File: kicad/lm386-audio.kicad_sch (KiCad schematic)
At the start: 34 parts, among them J3 Gain, J4 Audio_IN, J5 USB, J6 Headphones, M1 TP4056_MODULE, Q1 AO3407, U1 LM386, U2 SD6271 Step Up

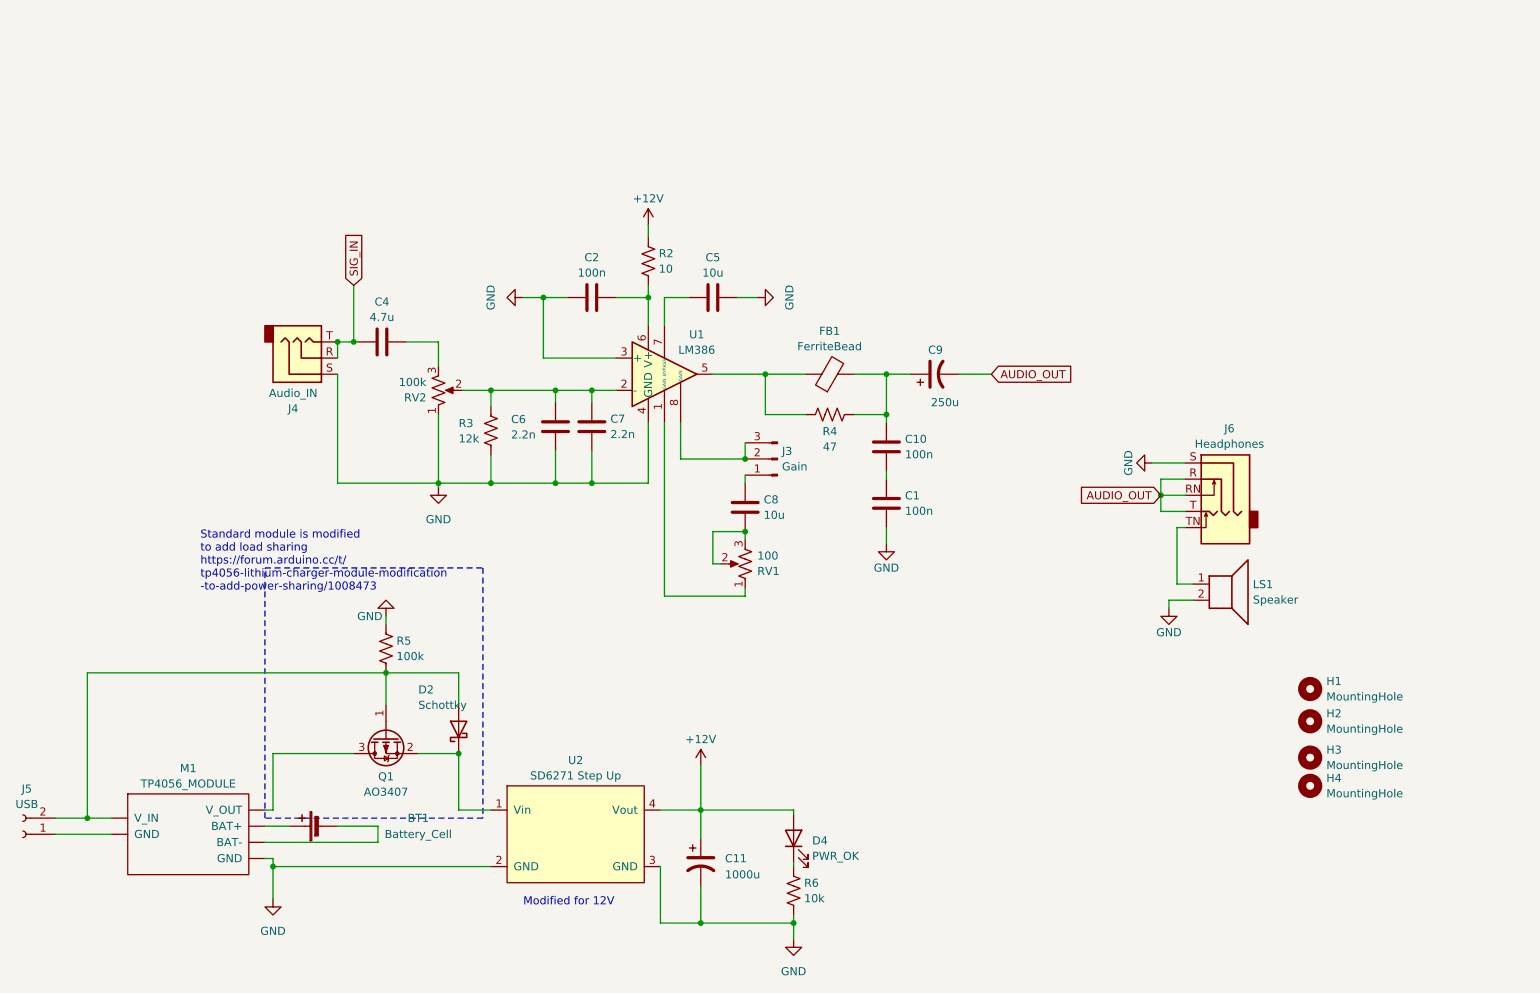
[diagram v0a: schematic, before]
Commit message: clean up + documentation
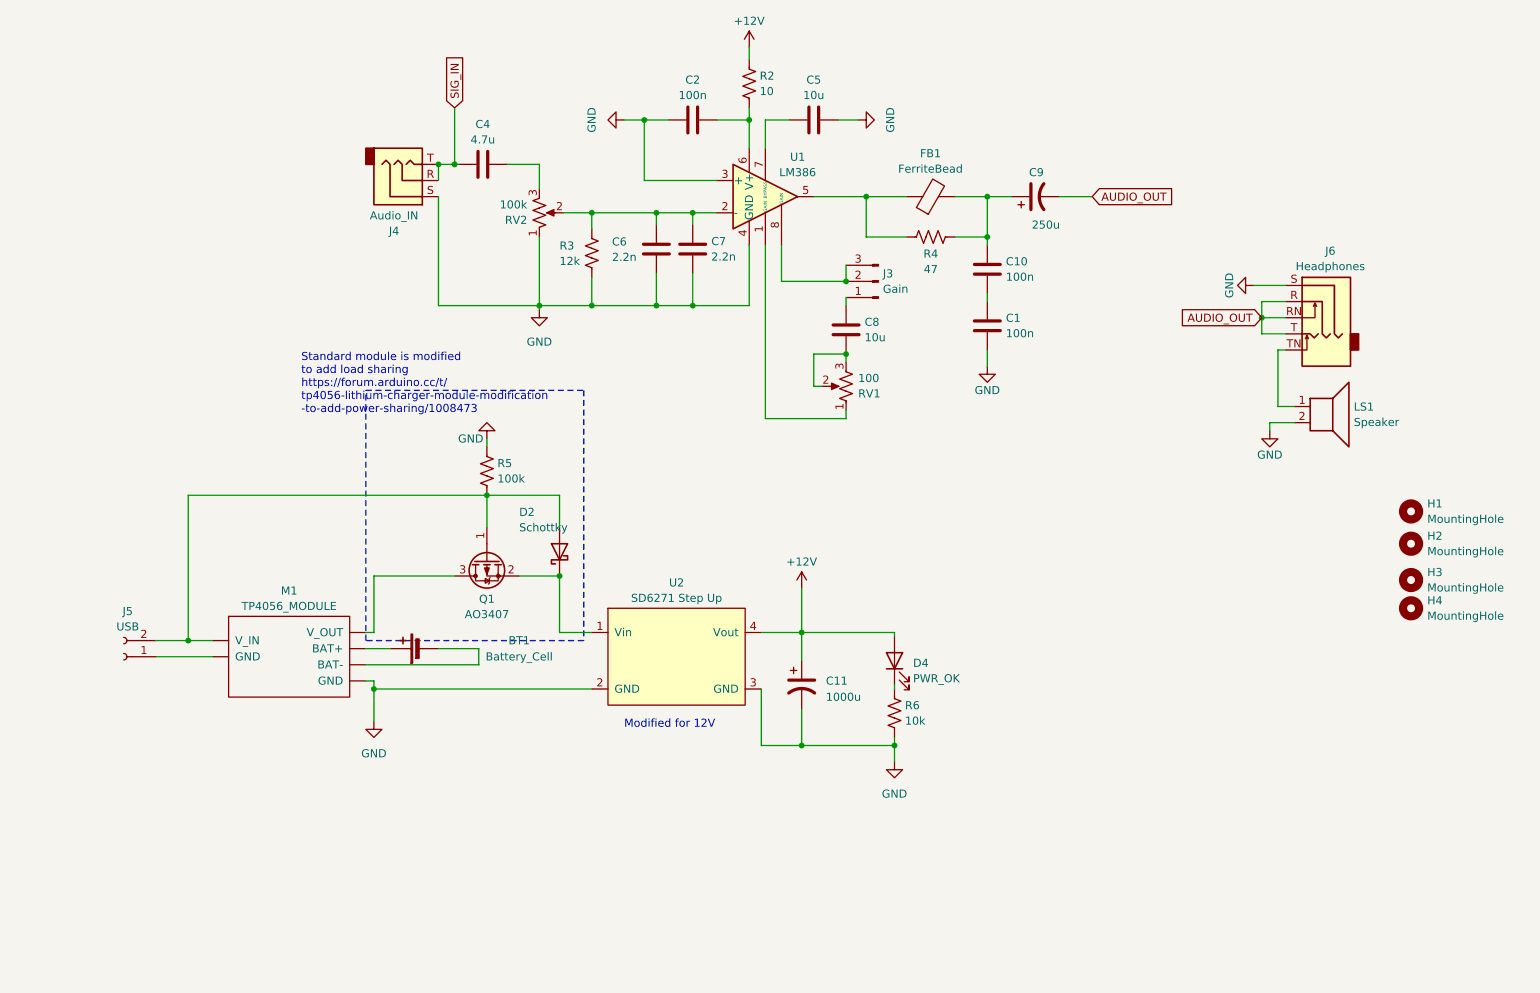
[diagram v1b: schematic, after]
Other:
- moved on the sheet: BT1, C1, C10, C11, C2, C4, C5, C6, C7, C8, C9, D2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
